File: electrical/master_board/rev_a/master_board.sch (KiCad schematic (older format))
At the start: 4 parts

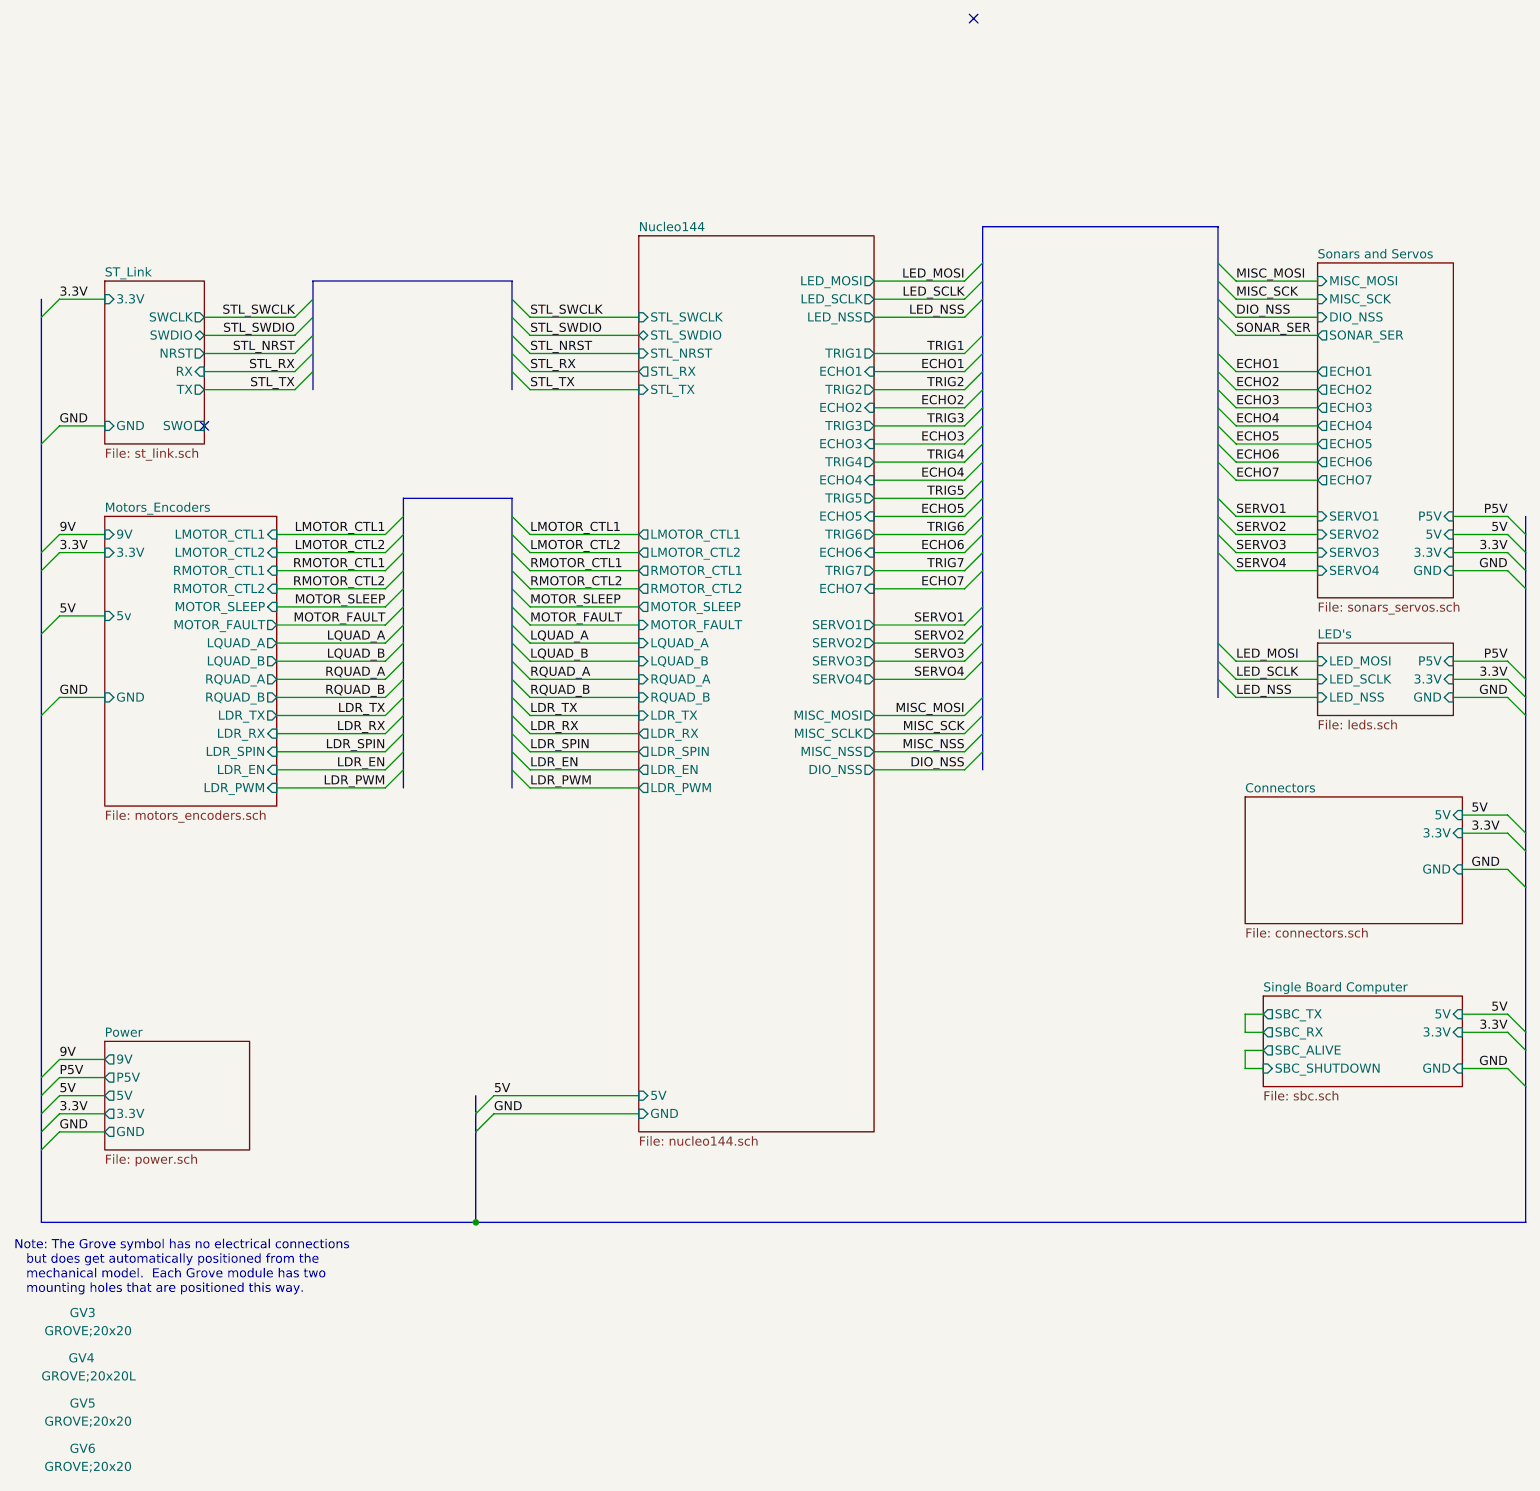
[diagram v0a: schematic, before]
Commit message: Lot's schematic work.
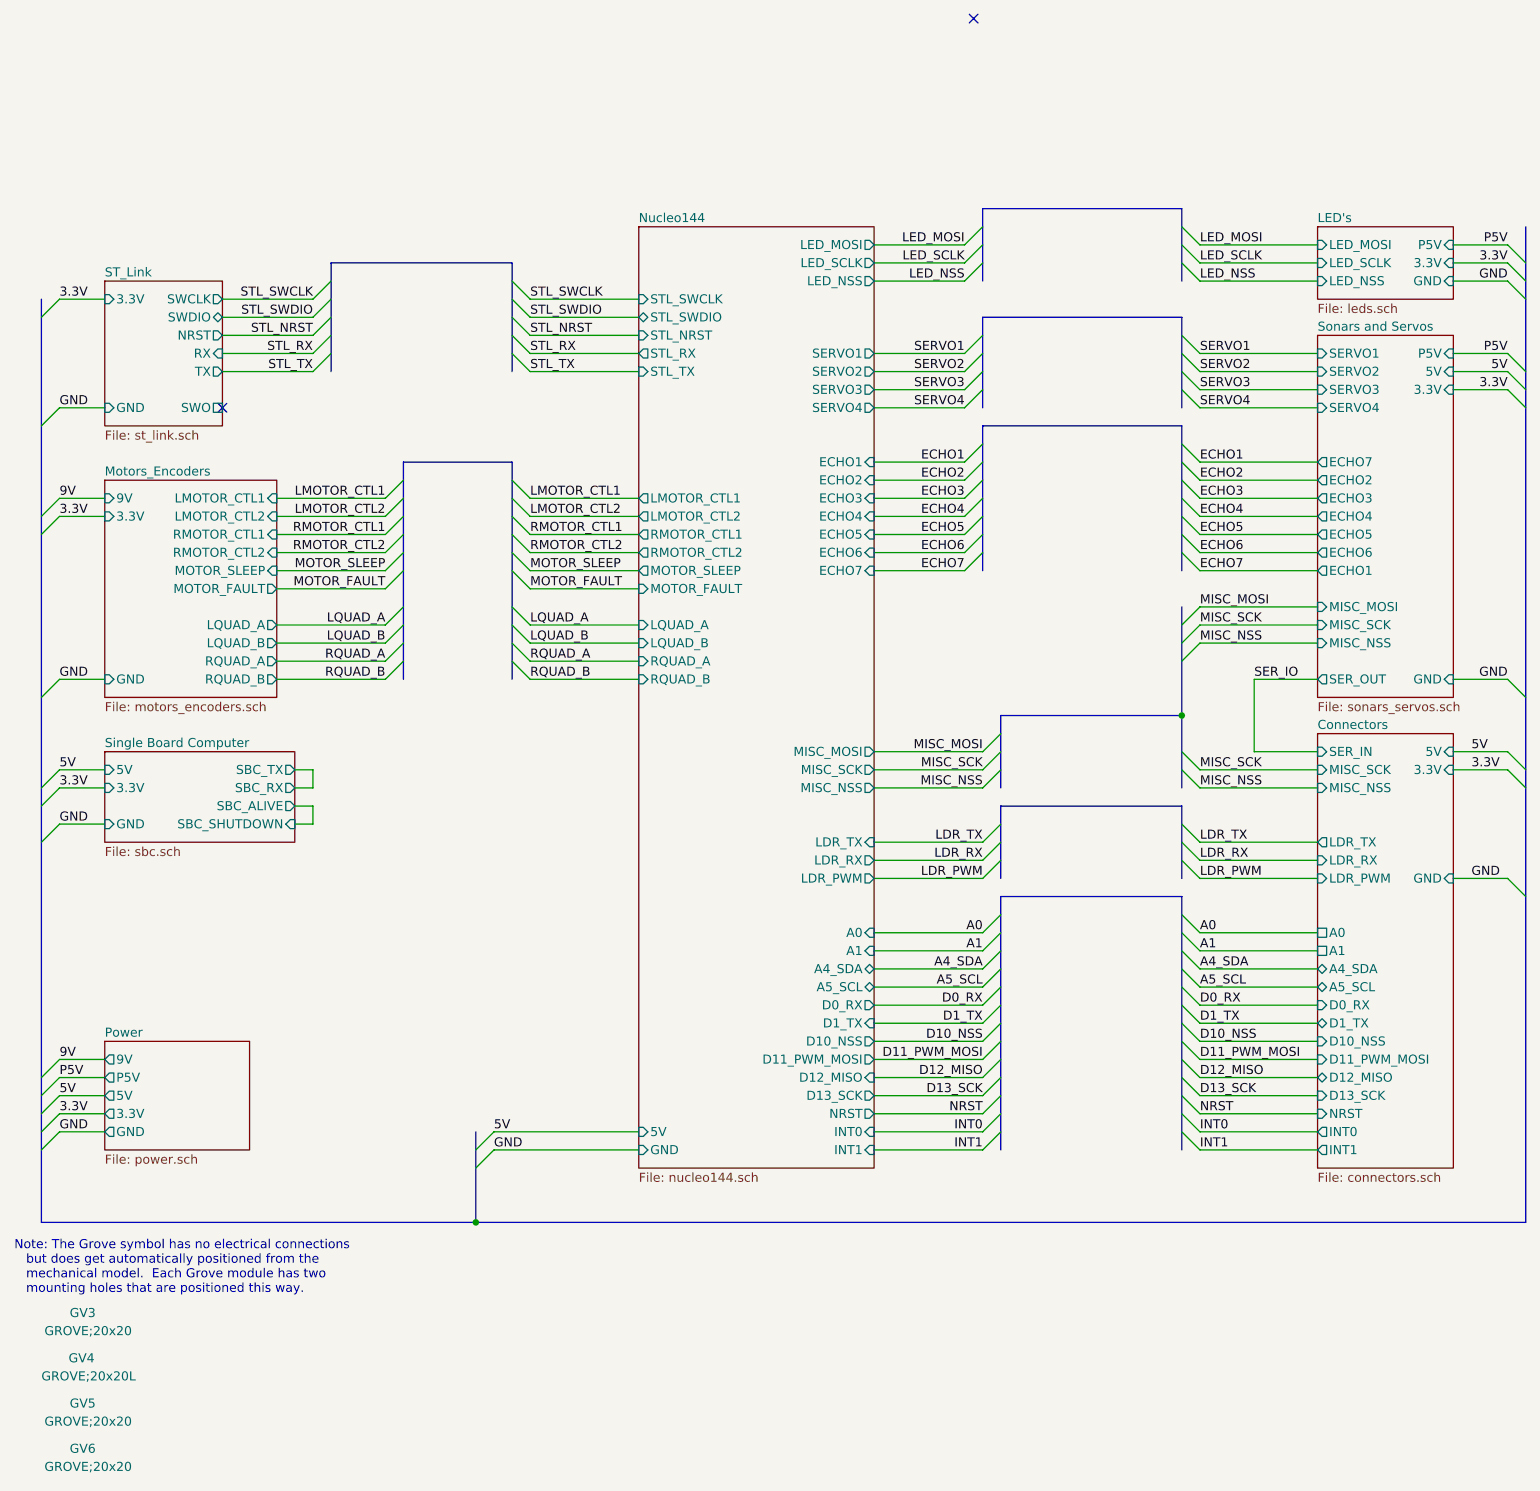
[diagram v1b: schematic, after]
